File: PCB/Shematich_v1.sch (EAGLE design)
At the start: 9 parts, among them U1 EK-TM4C123GXL, U2 4N25, X1 HD44780LCD-1602, X2 22-23-2081, X3 22-23-2031

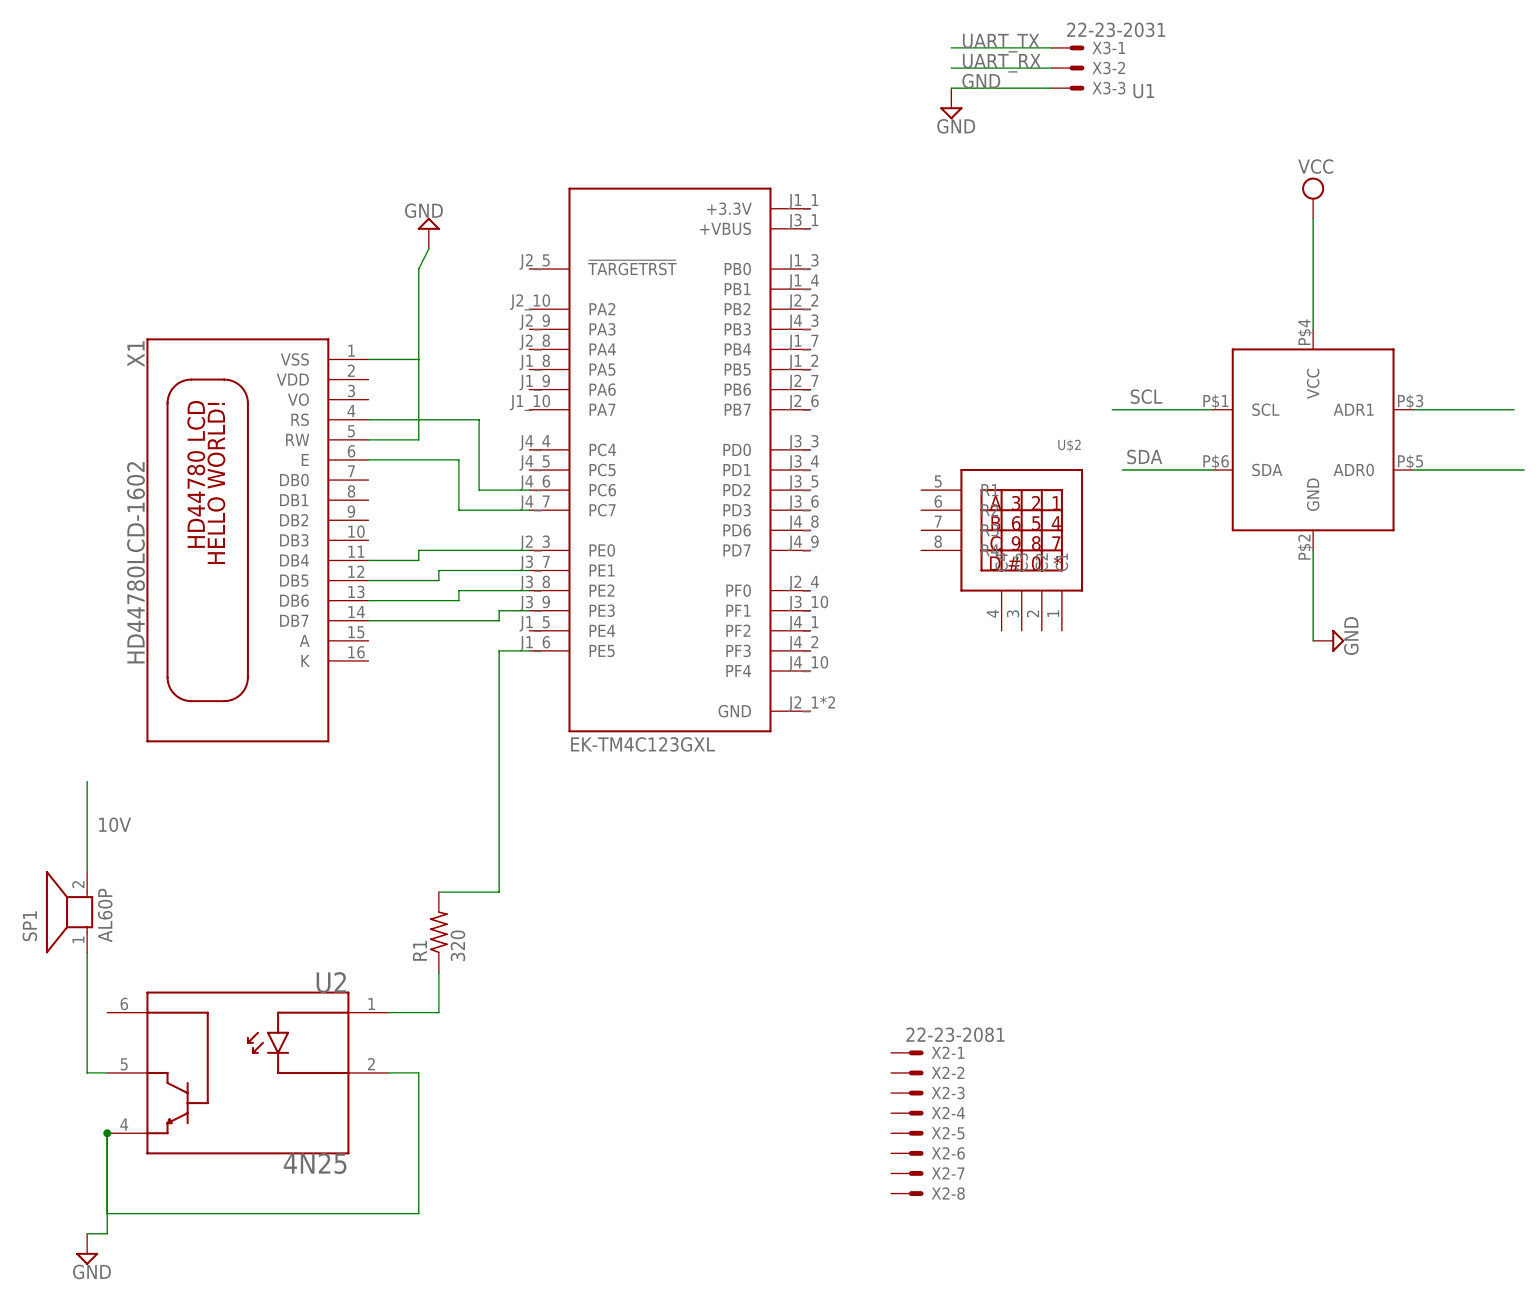
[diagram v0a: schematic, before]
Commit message: final schematic
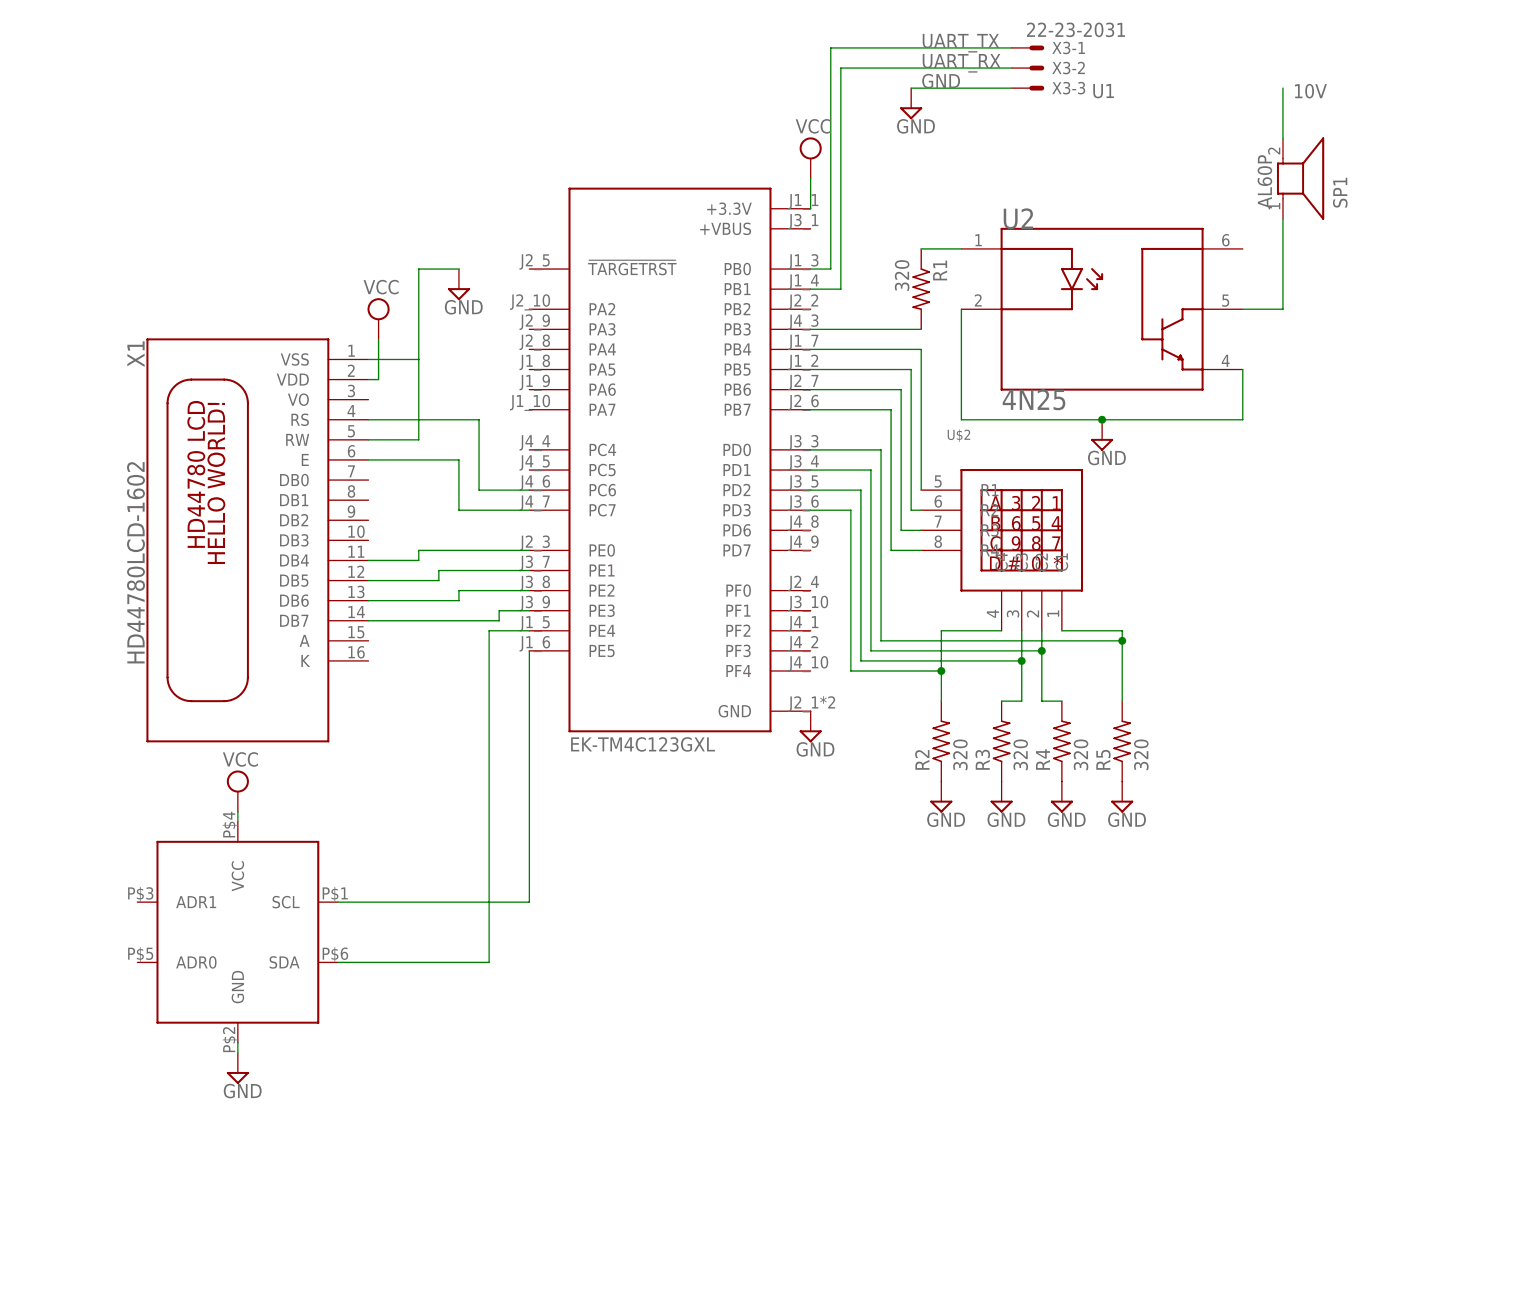
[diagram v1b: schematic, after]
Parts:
- removed X2: 22-23-2081, con-molex:22-23-2081
- added R2, R3, R4, R5: 320, rcl:R-US_0204/7
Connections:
- removed net N$11 (its old number): R1.2, U1.PE5
- removed net SCL: U$1.SCL
- removed net SDA: U$1.SDA
- new net N$1: R1.2, U1.PB3
- new net N$13: R2.2, U$2.C4, U1.PD3
- new net N$14: R4.2, U$2.C2, U1.PD1
- new net N$16: U$2.R1, U1.PB4
- new net N$17: U$2.R2, U1.PB5
- new net N$18: U$2.R3, U1.PB6
- new net N$19: U$2.R4, U1.PB7
- new net N$20: R5.2, U$2.C1, U1.PD0
- new net N$3: R3.2, U$2.C3, U1.PD2
- new net VDD: X1.VDD
- net GND: now also R2.1, R3.1, R4.1, R5.1, U1.GND
- net N$4: now also U$1.SCL, U1.PE5; no longer U$1.ADR0
- net N$5: now also U$1.SDA, U1.PE4; no longer U$1.ADR1
- net UART_RX: now also U1.PB1
- net UART_TX: now also U1.PB0
- net VCC: now also U1.+3.3V
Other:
- moved on the sheet: R1, SP1, U2, X3-1, X3-2, X3-3
